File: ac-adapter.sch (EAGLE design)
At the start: 67 parts, among them IC1 BM1Q011, IC2 TL431, Q1 TLP621-1, Q2 600V5A, T1 COMMON_FILTER-SU10VFC, T2 TRANSFORMAER_FLYBACK-PQ2620-2

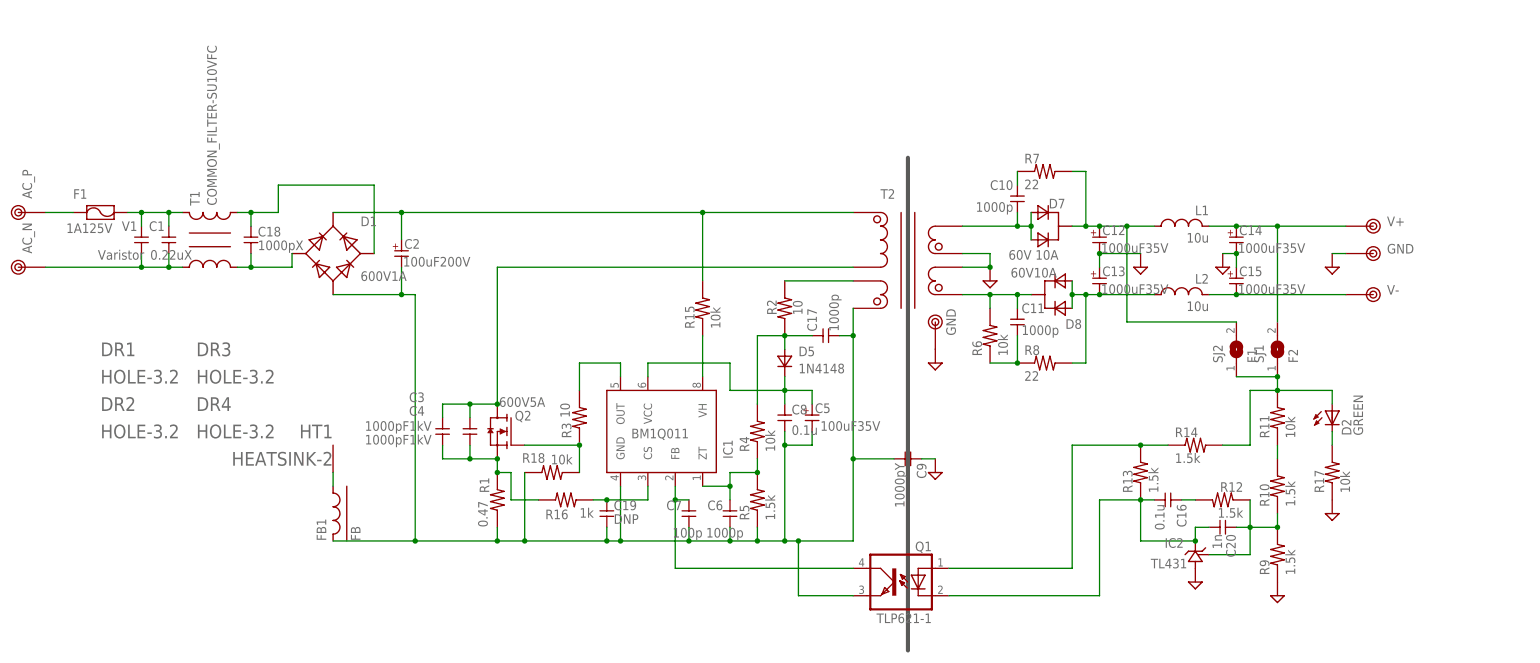
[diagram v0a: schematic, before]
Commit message: GaN
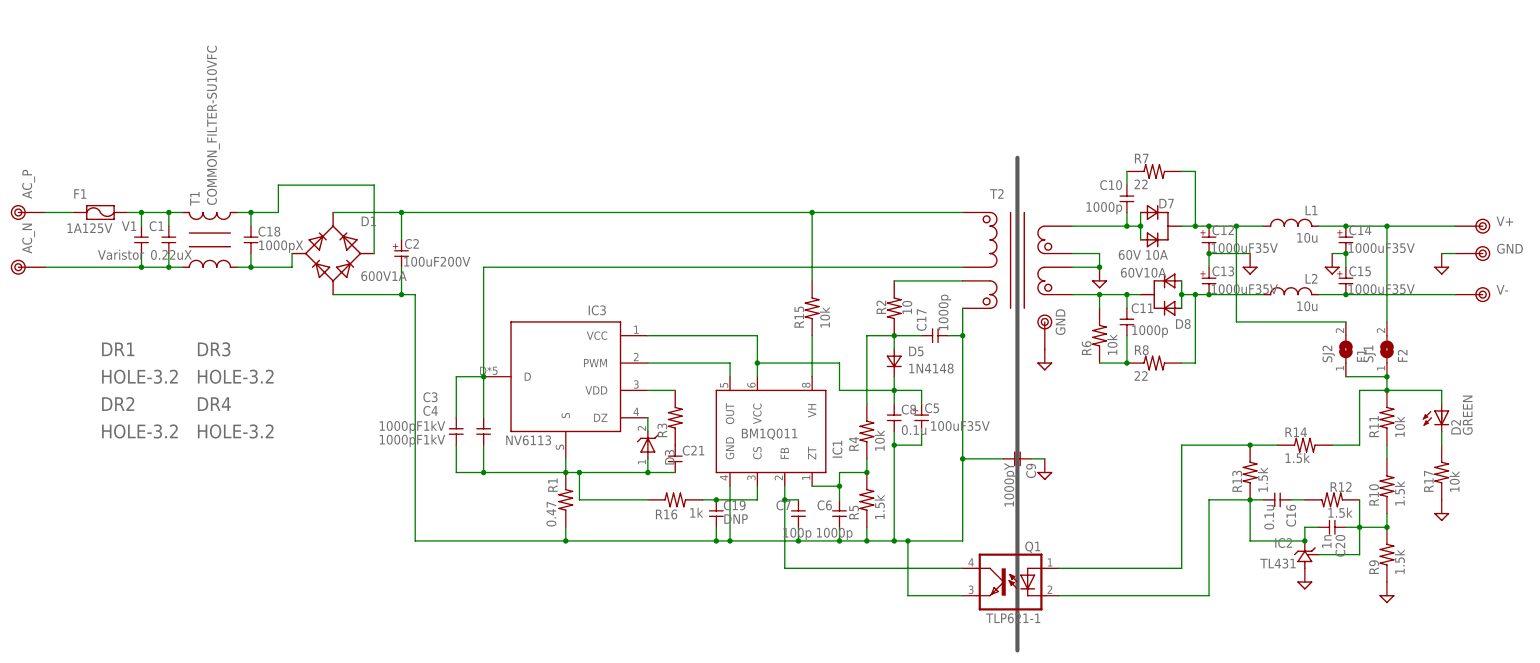
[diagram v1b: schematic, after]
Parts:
- removed FB1: FB, my_rcl:FB
- removed HT1: HEATSINK-2, my_connector:HEATSINK-2
- removed Q2: 600V5A, my_ic:NMOS
- removed R18: 10k, my_rcl:R-1608
- added C21: (no value), my_rcl:C-1608
- added D3: (no value), my_rcl:ZENER-SMD
- added IC3: NV6113, my_ic:NV6113
- R3: value 10 -> (none); device my_rcl:R-2012 -> my_rcl:R-1608
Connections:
- new net N$24: D3.C, IC3.DZ
- net N$12: now also C21.2, D3.A, IC3.S; no longer Q2.S
- net N$13: now also IC3.PWM; no longer R3.2
- net N$14: now also C21.1; no longer Q2.G, R18.1
- net N$20: now also IC3.VDD, R3.2; no longer FB1.1, HT1.HT
- net PGND: no longer FB1.2, R18.2
- net SW: now also IC3.D; no longer Q2.D
- net VCC: now also IC3.VCC
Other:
- moved on the sheet: C10, C11, C12, C13, C14, C15, C16, C17, C19, C20, C3, C4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
